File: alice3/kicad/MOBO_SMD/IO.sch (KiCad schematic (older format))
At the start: 36 parts, among them CON1 MicroSD, P2 USB_OTG, P3 UART1, SW2 SOFT RESET, U5 STM32F415RG, Y2 16MHz, Y3 32.768KHz

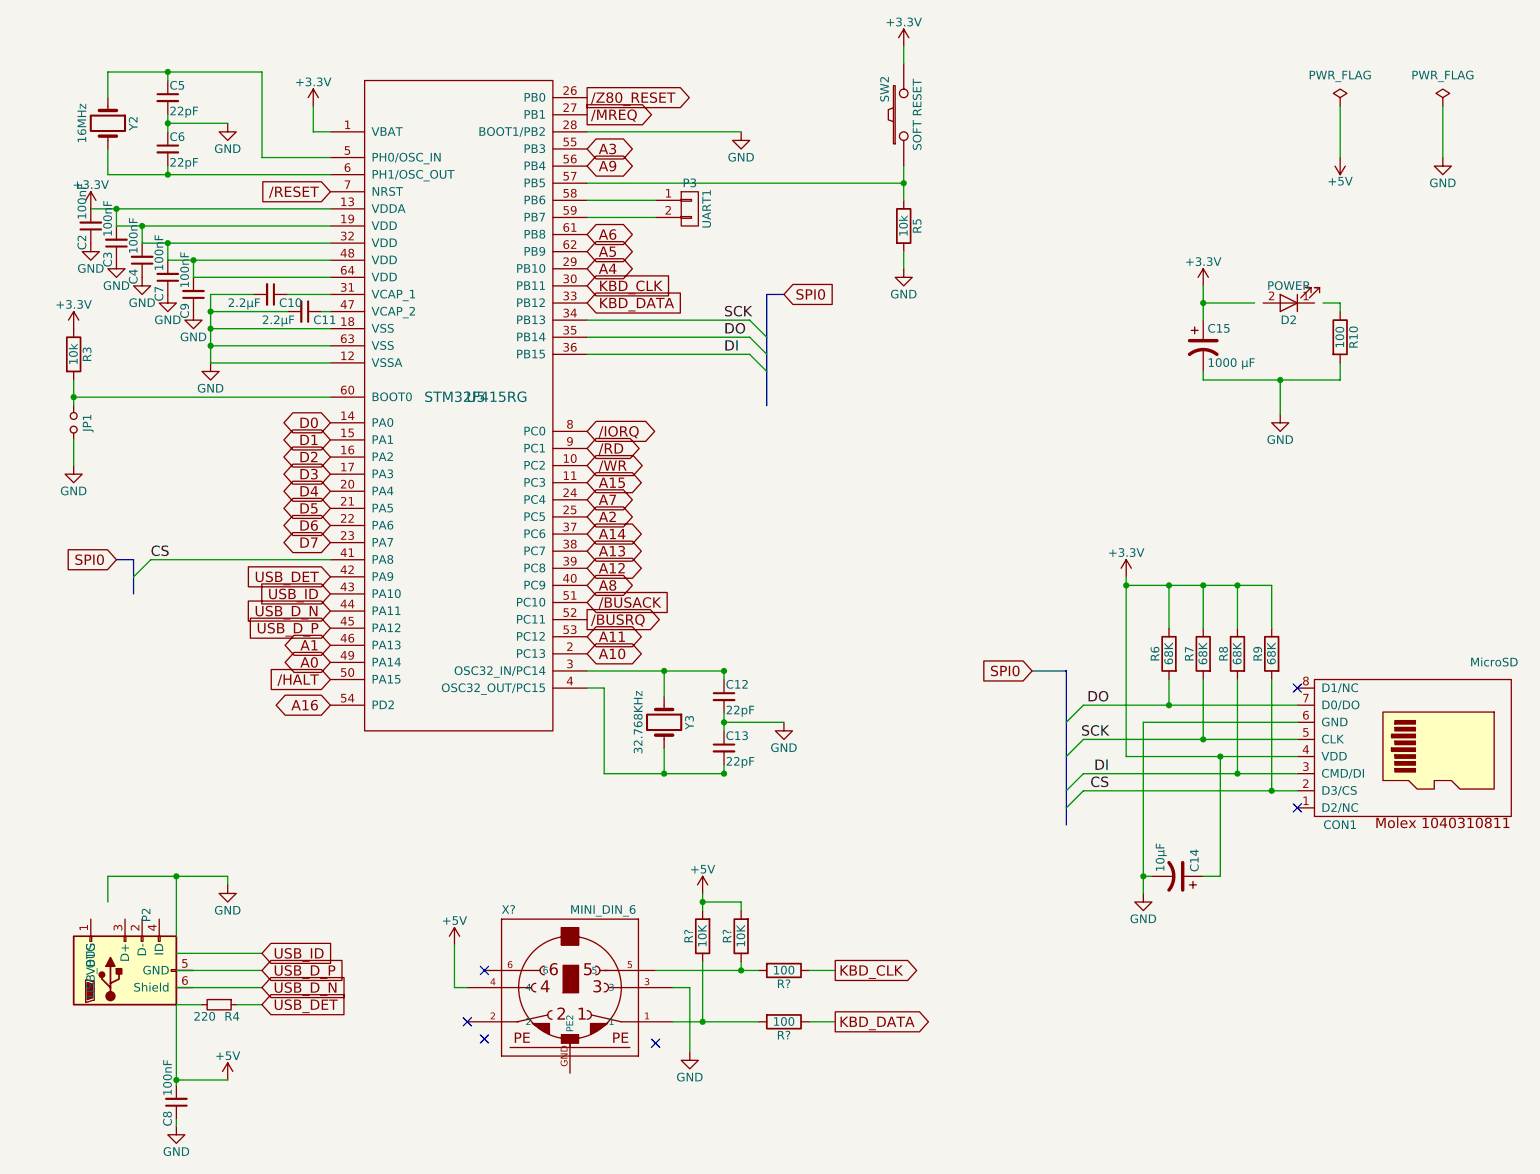
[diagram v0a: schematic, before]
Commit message: Fix up various small things.
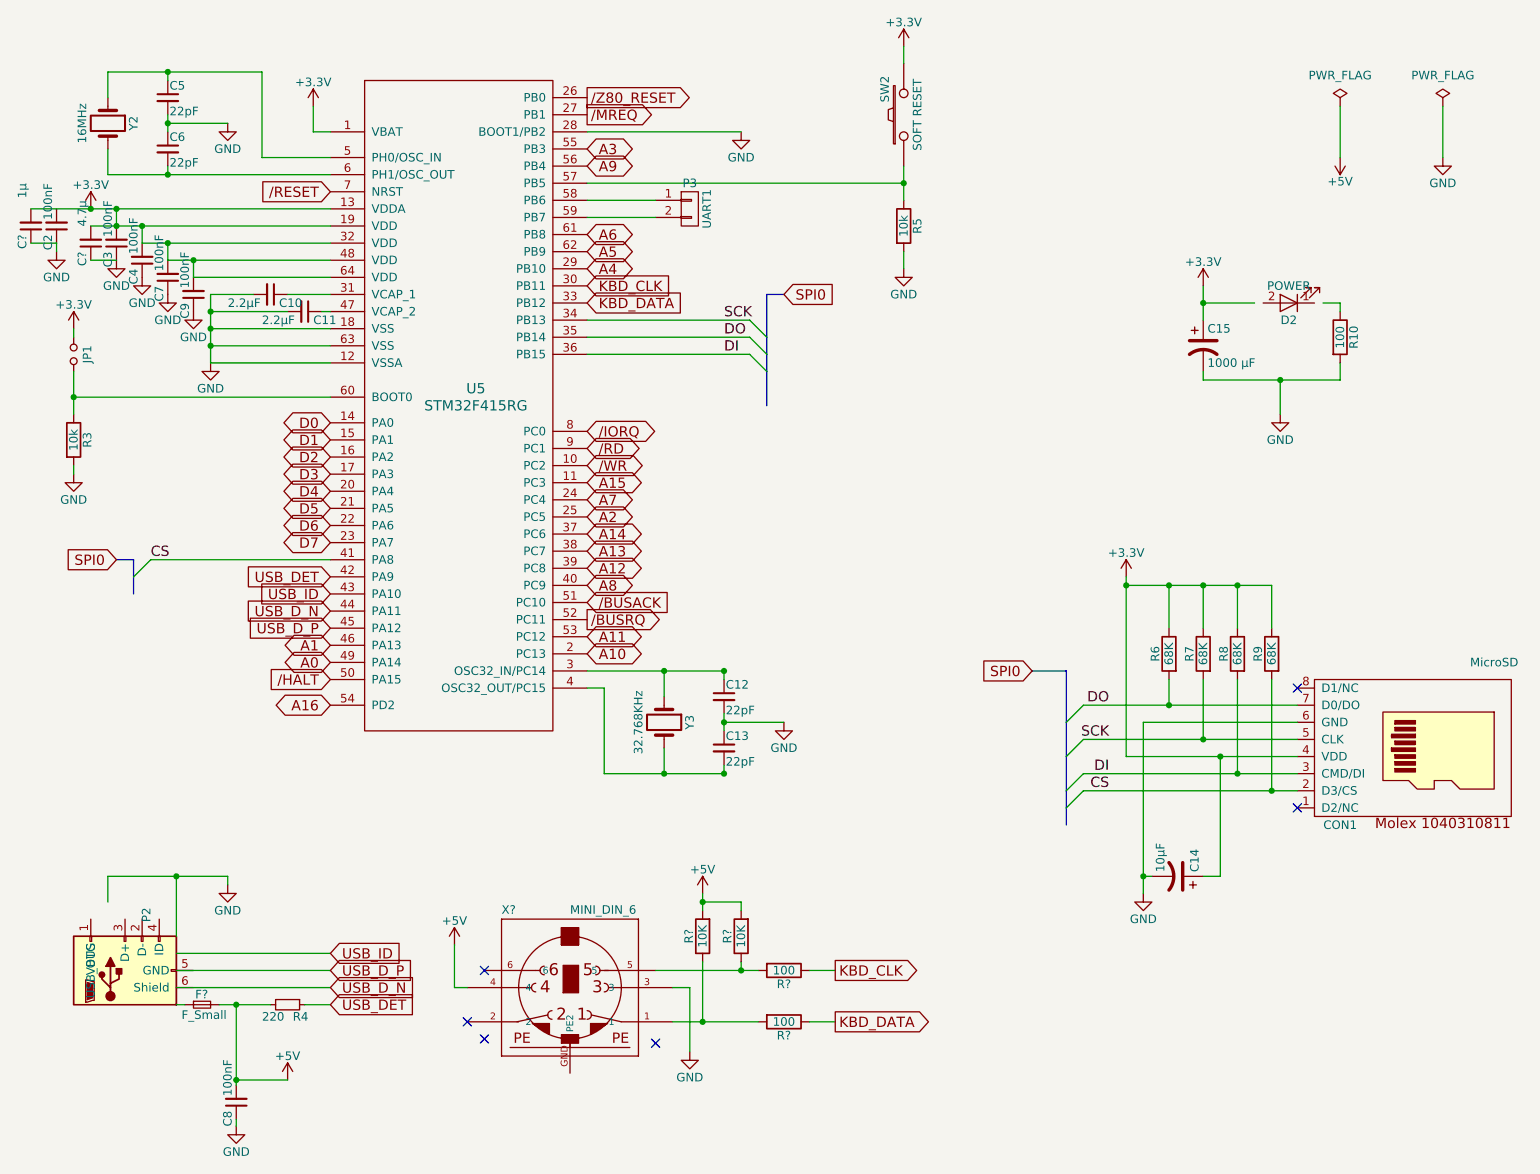
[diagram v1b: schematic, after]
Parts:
- added C?: 1µ, Capacitors_SMD:C_0805, symbol C_Small
- added C?: 4.7µ, Capacitors_SMD:C_0805, symbol C_Small
- added F?: F_Small, symbol F_Small
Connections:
- wire segments 108 -> 148
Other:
- moved on the sheet: C2, C8, JP1, R3, R4
